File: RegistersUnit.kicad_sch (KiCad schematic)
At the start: 20 parts, among them U23 74LS139, U24 74LS139, U25 74LS08, U26 74LS00, U57 74LS377, U58 74LS541, U59 74LS377, U60 74LS541, U61 74LS377, U62 74LS377, U63 74LS541, U64 74LS541

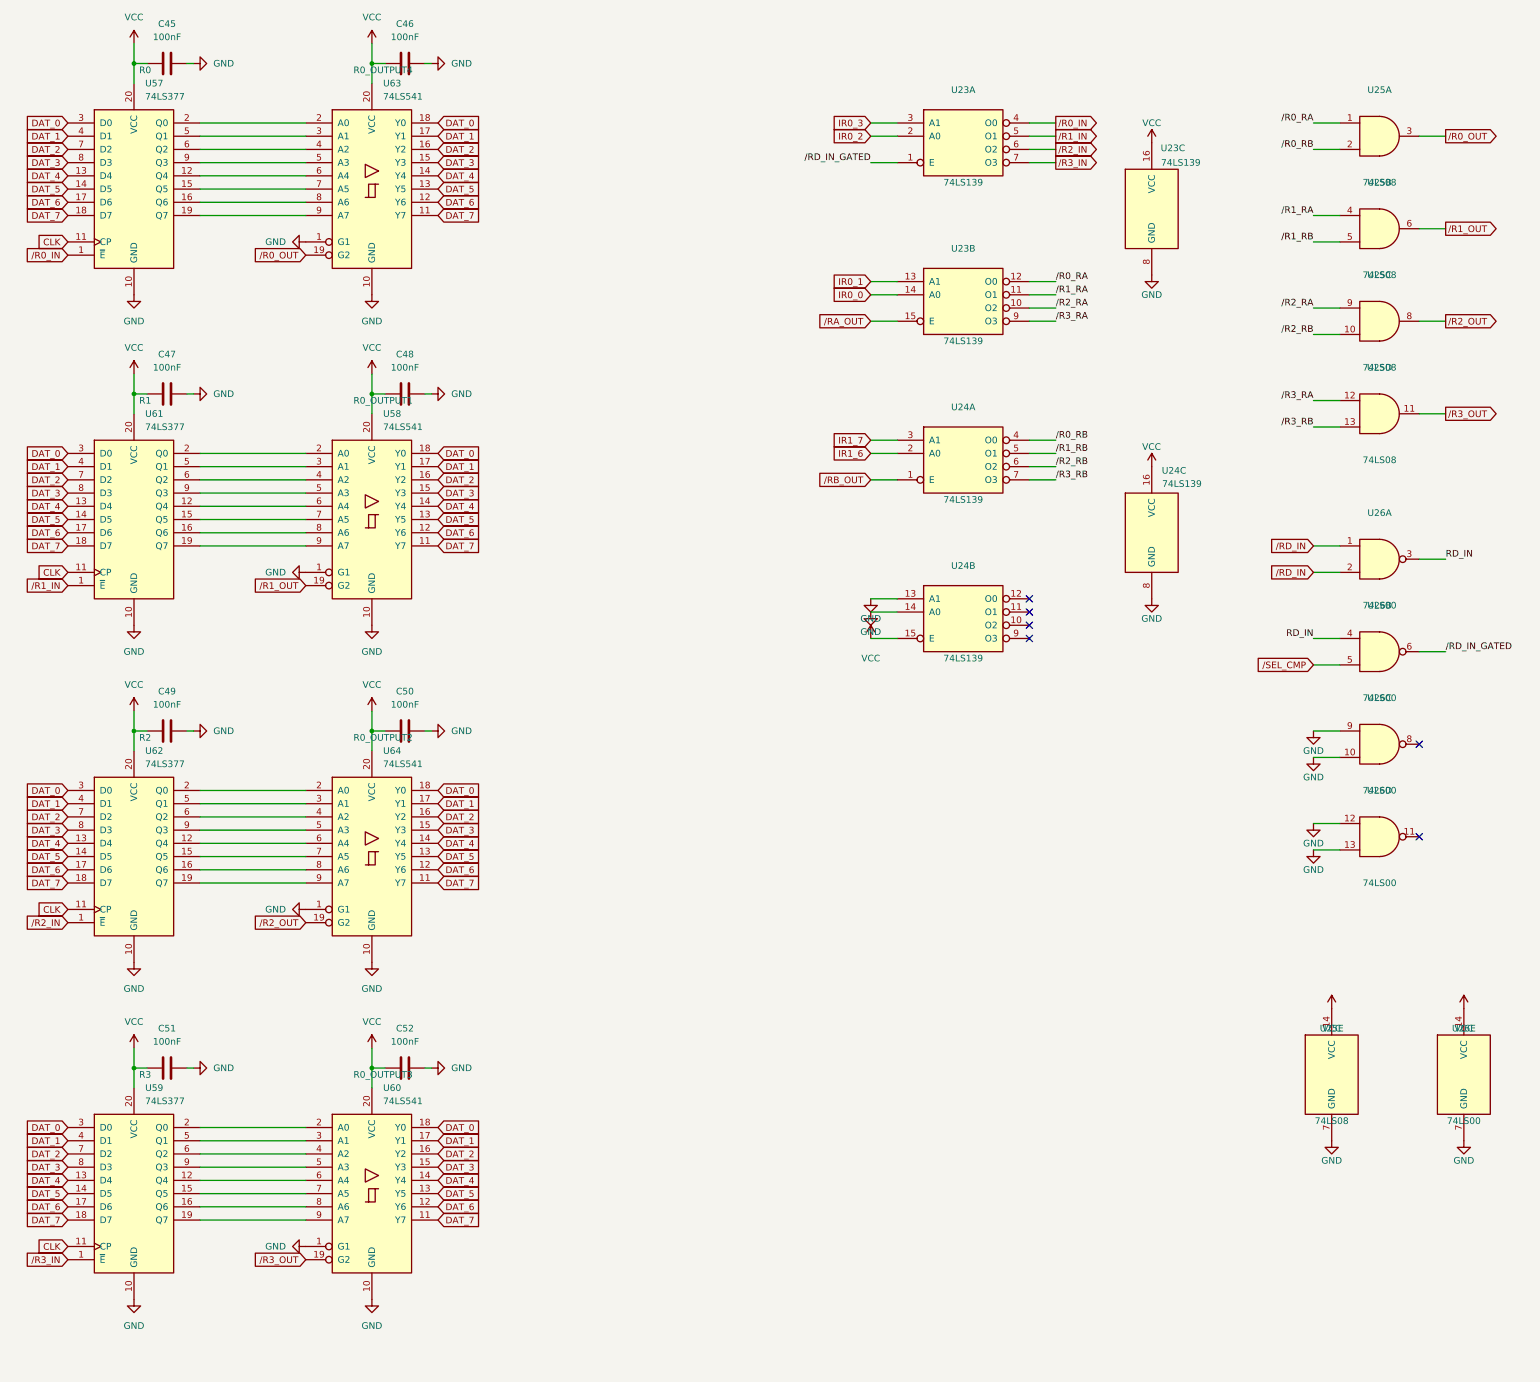
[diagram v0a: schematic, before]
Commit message: Fixes Gate symbol refs and adds backplane definition
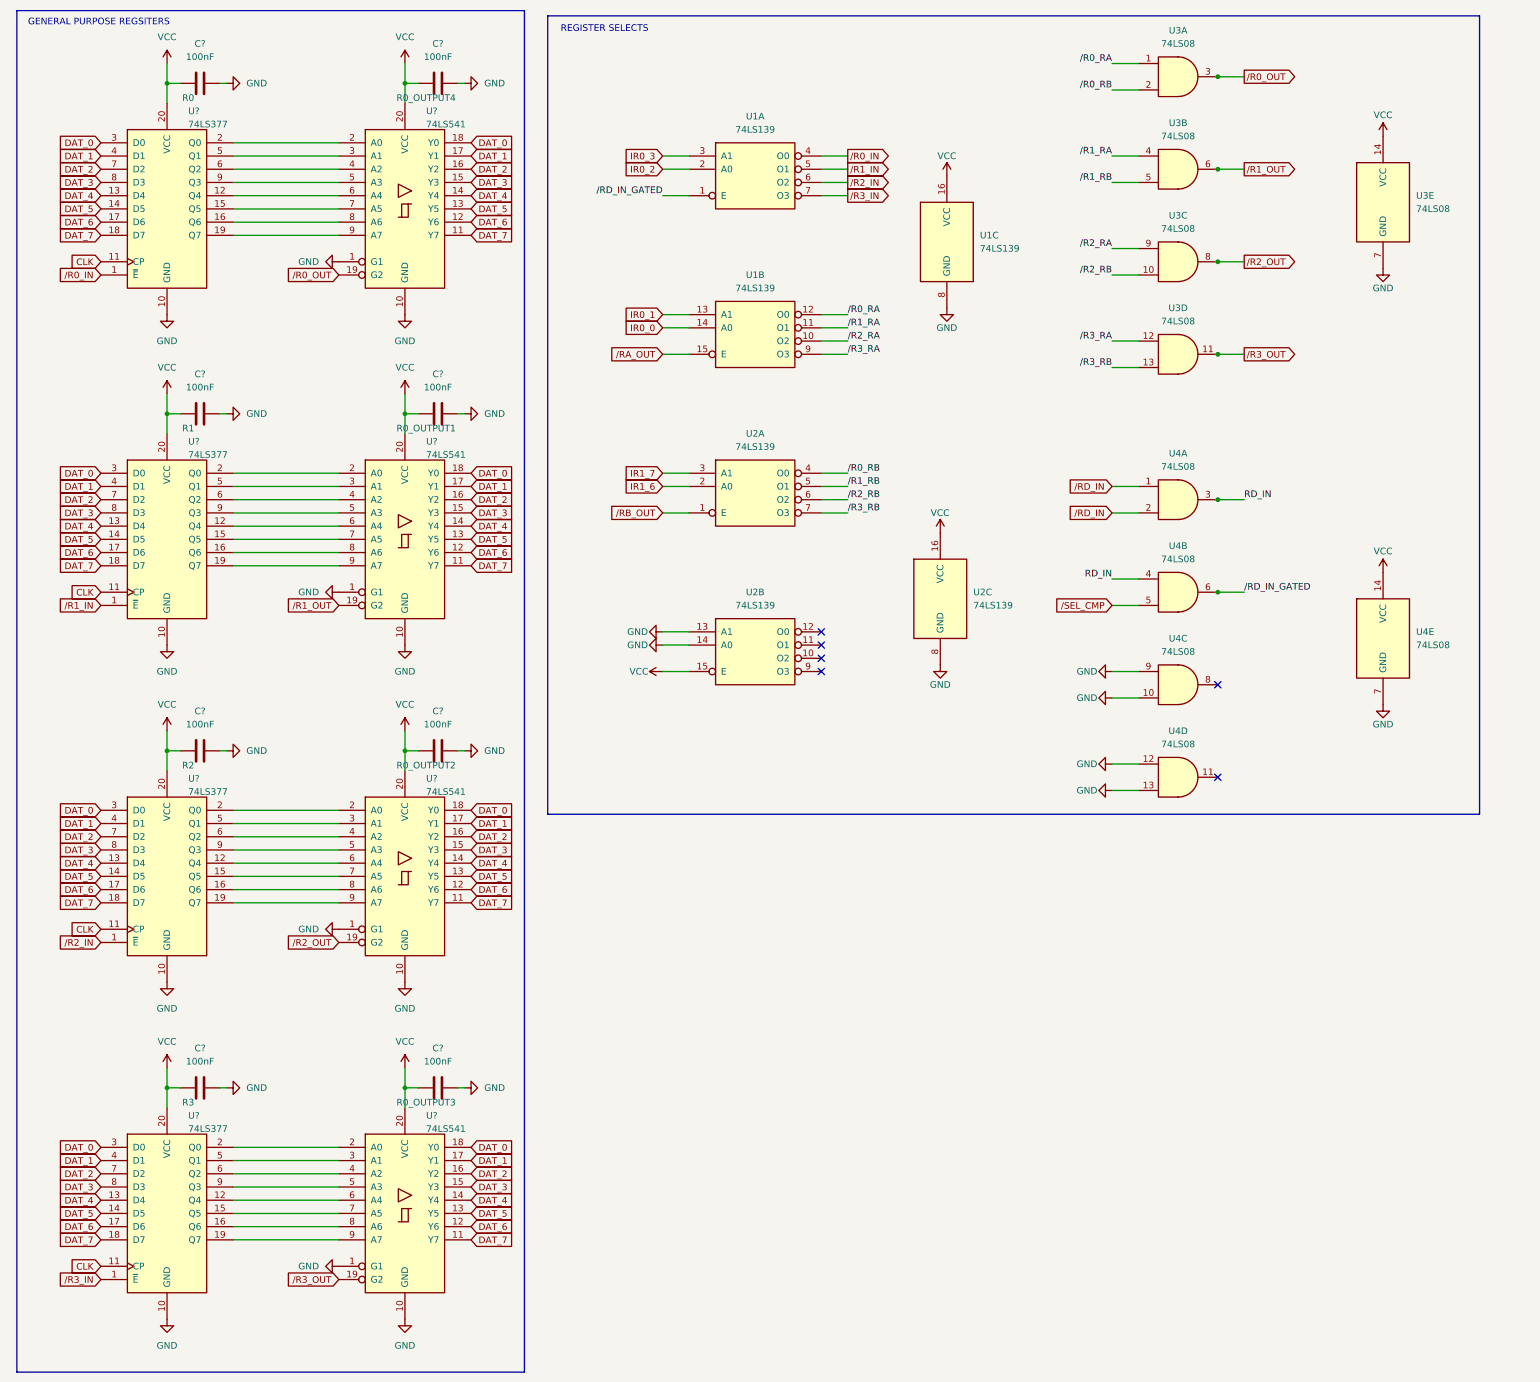
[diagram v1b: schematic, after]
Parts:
- removed U23, U24: 74LS139, Package_DIP:DIP-16_W7.62mm, symbol 74xx:74LS139
- removed U25: 74LS08, Package_DIP:DIP-14_W7.62mm, symbol 74xx:74LS08
- removed U26: 74LS00, Package_DIP:DIP-14_W7.62mm, symbol 74xx:74LS00
- added U1, U2: 74LS139, symbol 74xx:74LS139
- added U3, U4: 74LS08, symbol 74xx:74LS08
- renumbered C49 to C?, C45 to C?, C52 to C?, C51 to C?, C47 to C?, C50 to C?, C48 to C?, C46 to C?, U57 to U?, U58 to U?, U59 to U?, U60 to U?, U61 to U?, U62 to U?, U63 to U?, U64 to U?
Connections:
- net GND: now also U1.8 (GND), U2.13 (A1), U2.14 (A0), U2.8 (GND), U3.7 (GND), U4.7 (GND)
- net IR0_0: now also U1.14 (A0)
- net IR0_1: now also U1.13 (A1)
- net IR0_2: now also U1.2 (A0)
- net IR0_3: now also U1.3 (A1)
- net IR1_6: now also U2.2 (A0)
- net IR1_7: now also U2.3 (A1)
- net RD_IN: now also U4.3
- net VCC: now also U1.16 (VCC), U2.15 (E), U2.16 (VCC), U3.14 (VCC), U4.14 (VCC)
- net /R0_IN: now also U1.4 (O0)
- net /R0_OUT: now also U3.3
- net /R0_RA: now also U1.12 (O0)
- net /R0_RB: now also U2.4 (O0)
- net /R1_IN: now also U1.5 (O1)
- net /R1_OUT: now also U3.6
- net /R1_RA: now also U1.11 (O1)
- net /R1_RB: now also U2.5 (O1)
- net /R2_IN: now also U1.6 (O2)
- net /R2_OUT: now also U3.8
- net /R2_RA: now also U1.10 (O2)
- net /R2_RB: now also U2.6 (O2)
- net /R3_IN: now also U1.7 (O3)
- net /R3_OUT: now also U3.11
- net /R3_RA: now also U1.9 (O3)
- net /R3_RB: now also U2.7 (O3)
- net /RA_OUT: now also U1.15 (E)
- net /RB_OUT: now also U2.1 (E)
- net /RD_IN_GATED: now also U1.1 (E), U4.6
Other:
- note added: "GENERAL PURPOSE REGSITERS"
- note added: "REGISTER SELECTS"
- moved on the sheet: C?, U?
